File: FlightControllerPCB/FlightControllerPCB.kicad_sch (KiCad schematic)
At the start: 0 parts

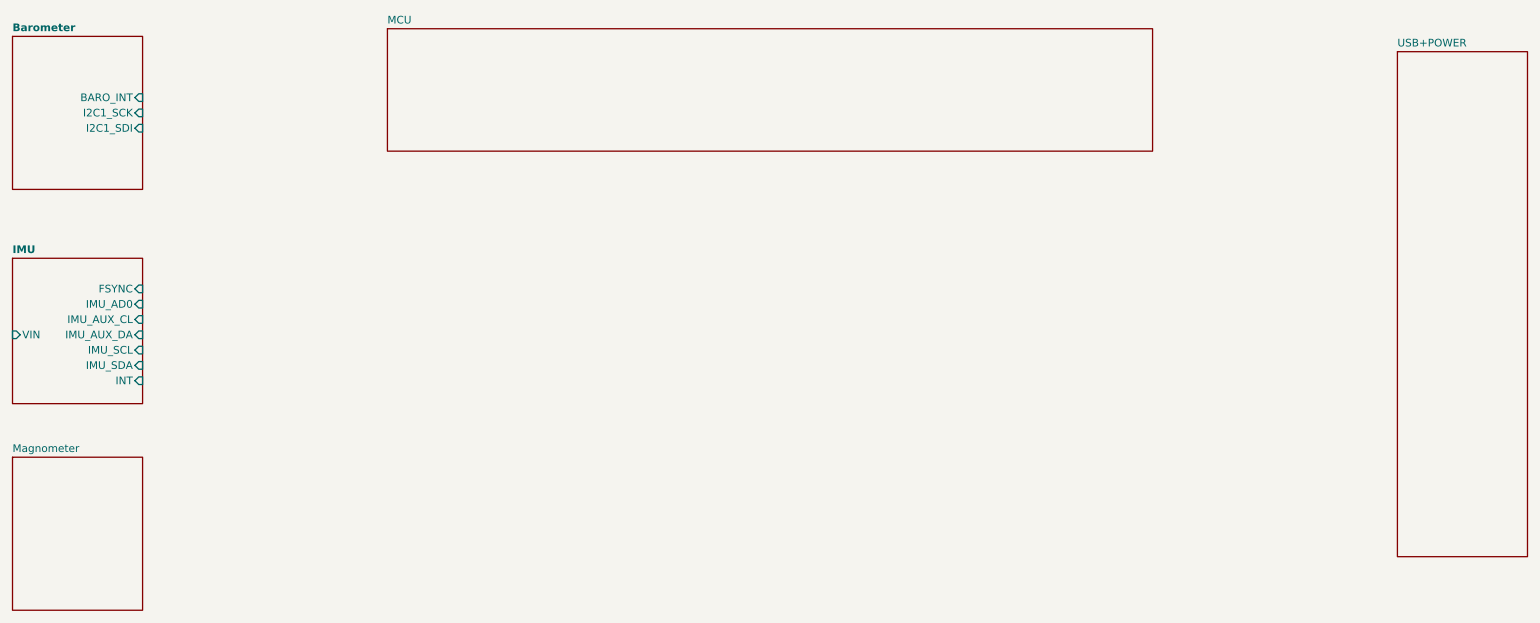
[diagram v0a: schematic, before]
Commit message: Early MCU Setup
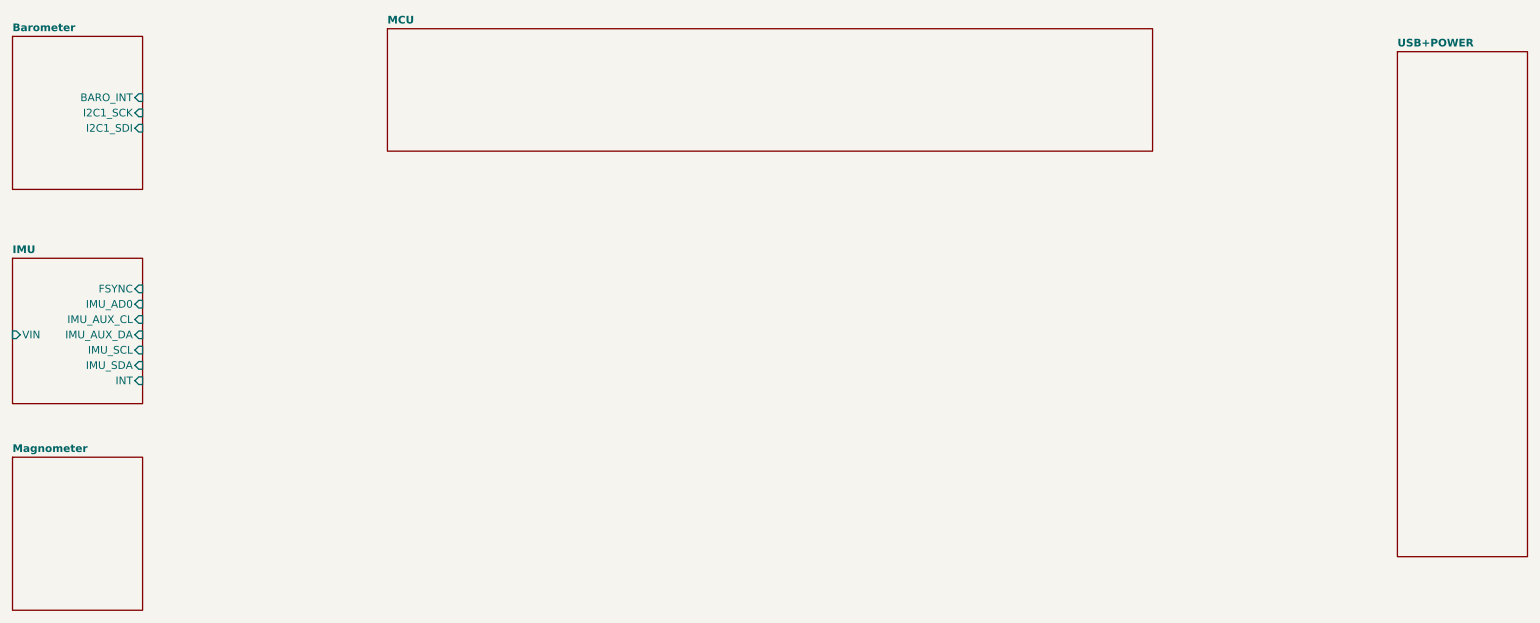
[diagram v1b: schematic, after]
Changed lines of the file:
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@@
 				(font
 					(size 1.27 1.27)
+					(thickness 0.254)
+					(bold yes)
 				)
 				(justify left bottom)
@@
 				(font
 					(size 1.27 1.27)
+					(thickness 0.254)
+					(bold yes)
 				)
 				(justify left bottom)
@@
 				(font
 					(size 1.27 1.27)
-				)
-				(justify left bottom)
+					(thickness 0.254)
+					(bold yes)
+				)
+				(justify left bottom)
